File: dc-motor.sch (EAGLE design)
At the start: 82 parts, among them IC1 MEGA32-A, X3 RIA_3POL, X4 RIA_3POL, X5 RIA_2POL, X6 JUMP1-4, X8 PFVERB10

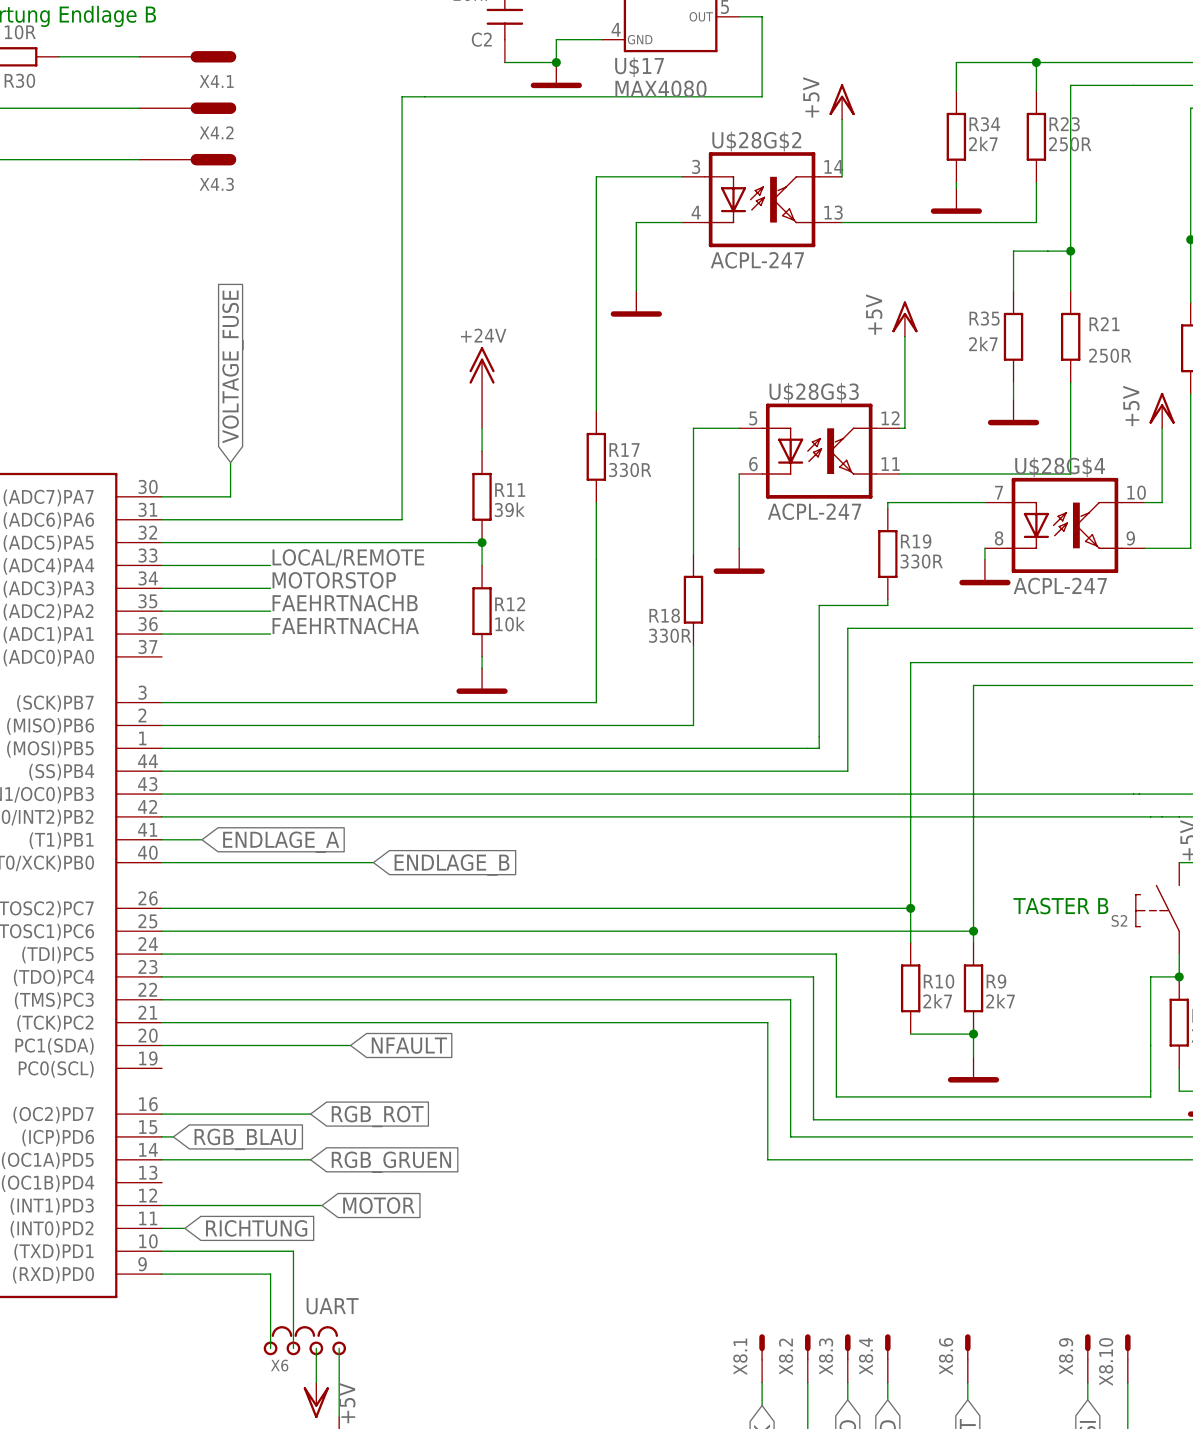
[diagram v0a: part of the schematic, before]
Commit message: edited again
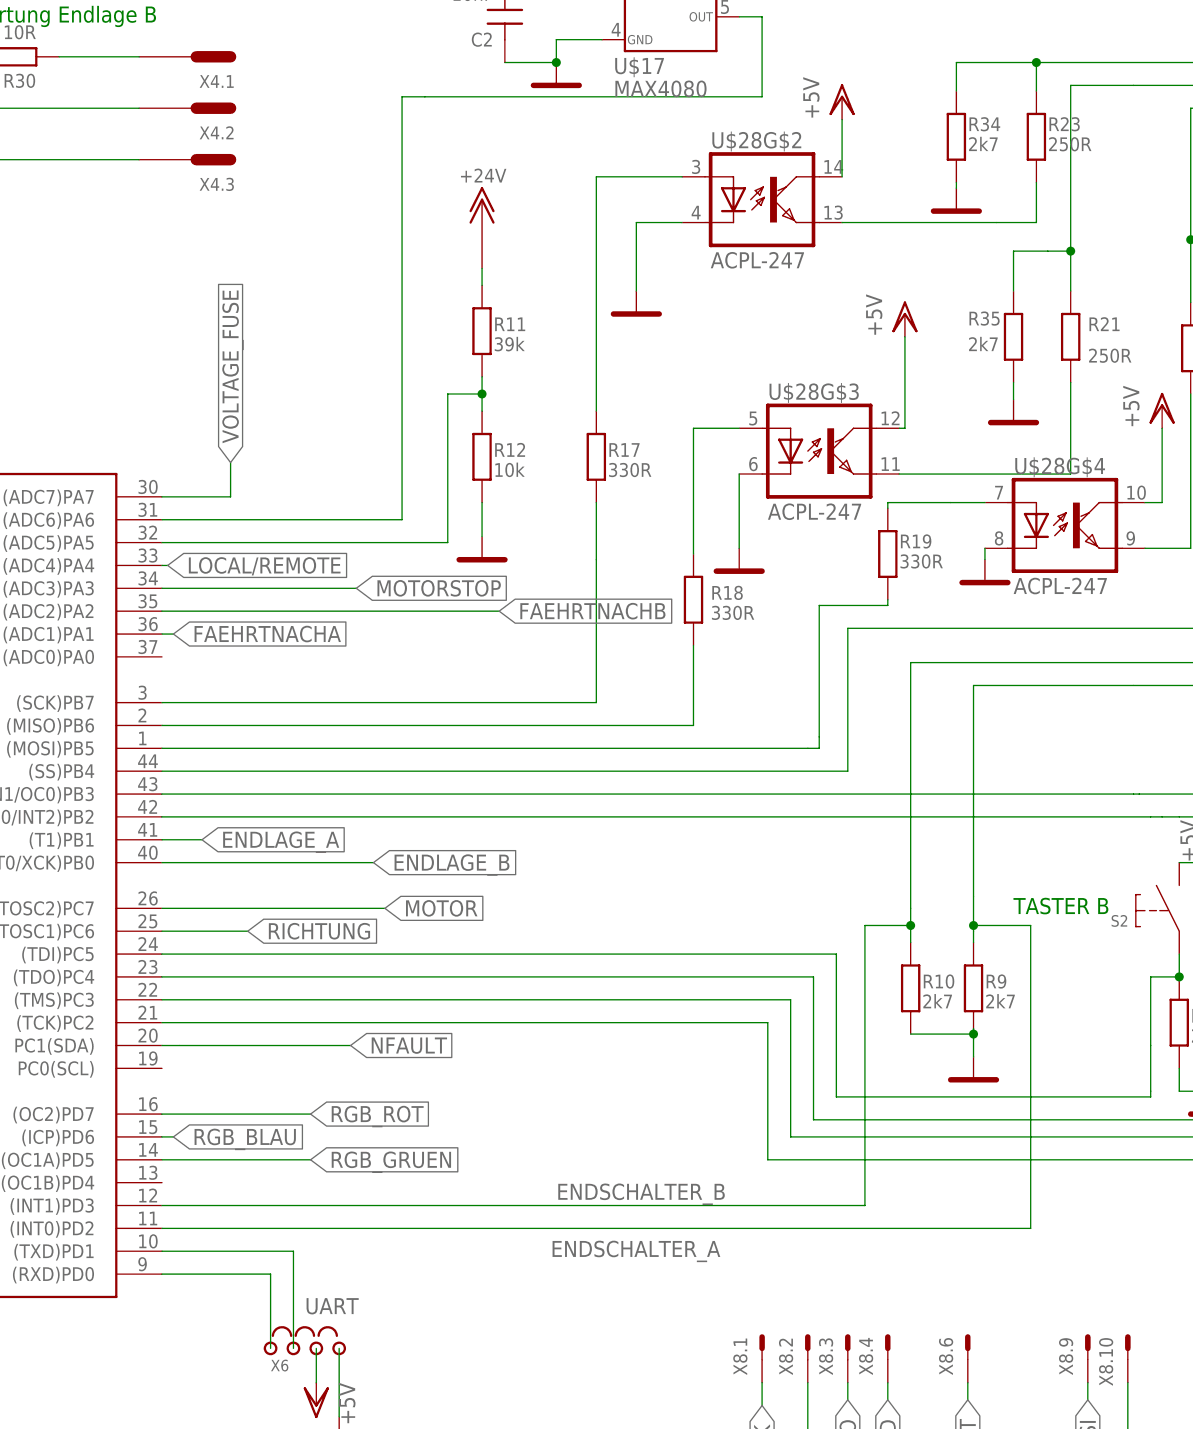
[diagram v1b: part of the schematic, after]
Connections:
- net ENDSCHALTER_A: now also IC1.(INT0)PD2; no longer IC1.(TOSC1)PC6
- net ENDSCHALTER_B: now also IC1.(INT1)PD3; no longer IC1.(TOSC2)PC7
- net MOTOR: now also IC1.(TOSC2)PC7; no longer IC1.(INT1)PD3
- net RICHTUNG: now also IC1.(TOSC1)PC6; no longer IC1.(INT0)PD2
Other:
- moved on the sheet: R11, R12
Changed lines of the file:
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@@
 </instance>
 <instance part="U$25" gate="G$1" x="288.29" y="191.135"/>
-<instance part="R11" gate="G$1" x="141.605" y="127" smashed="yes" rot="R90">
-<attribute name="NAME" x="142.875" y="127" size="1.524" layer="95"/>
-<attribute name="VALUE" x="142.875" y="124.7775" size="1.524" layer="96"/>
-</instance>
-<instance part="R12" gate="G$1" x="141.605" y="114.3" smashed="yes" rot="R90">
-<attribute name="NAME" x="142.875" y="114.3" size="1.524" layer="95"/>
-<attribute name="VALUE" x="142.875" y="112.0775" size="1.524" layer="96"/>
-</instance>
-<instance part="U$26" gate="G$1" x="141.605" y="105.41"/>
-<instance part="U$27" gate="G$1" x="141.605" y="137.16"/>
+<instance part="R11" gate="G$1" x="141.605" y="145.415" smashed="yes" rot="R90">
+<attribute name="NAME" x="142.875" y="145.415" size="1.524" layer="95"/>
+<attribute name="VALUE" x="142.875" y="143.1925" size="1.524" layer="96"/>
+</instance>
+<instance part="R12" gate="G$1" x="141.605" y="131.445" smashed="yes" rot="R90">
+<attribute name="NAME" x="142.875" y="131.445" size="1.524" layer="95"/>
+<attribute name="VALUE" x="142.875" y="129.2225" size="1.524" layer="96"/>
+</instance>
+<instance part="U$26" gate="G$1" x="141.605" y="120.015"/>
+<instance part="U$27" gate="G$1" x="141.605" y="154.94"/>
 <instance part="R14" gate="G$1" x="307.975" y="181.61" smashed="yes" rot="R90">
 <attribute name="NAME" x="309.245" y="181.61" size="1.524" layer="95"/>
@@
 </instance>
 <instance part="R18" gate="G$1" x="165.1" y="115.57" smashed="yes" rot="R270">
-<attribute name="NAME" x="160.02" y="113.03" size="1.524" layer="95"/>
-<attribute name="VALUE" x="160.02" y="110.8075" size="1.524" layer="96"/>
+<attribute name="NAME" x="167.005" y="115.57" size="1.524" layer="95"/>
+<attribute name="VALUE" x="167.005" y="113.3475" size="1.524" layer="96"/>
 </instance>
 <instance part="R19" gate="G$1" x="186.69" y="120.65" smashed="yes" rot="R90">
@@
 <pinref part="R12" gate="G$1" pin="1"/>
 <pinref part="U$26" gate="G$1" pin="GND"/>
-<wire x1="141.605" y1="109.22" x2="141.605" y2="107.95" width="0.1524" layer="91"/>
+<wire x1="141.605" y1="126.365" x2="141.605" y2="122.555" width="0.1524" layer="91"/>
 </segment>
 <segment>
@@
 <segment>
 <pinref part="R11" gate="G$1" pin="2"/>
-<wire x1="141.605" y1="132.08" x2="141.605" y2="134.62" width="0.1524" layer="91"/>
+<wire x1="141.605" y1="150.495" x2="141.605" y2="152.4" width="0.1524" layer="91"/>
 <pinref part="U$27" gate="G$1" pin="+24V"/>
 </segment>
@@
 <pinref part="R9" gate="G$1" pin="2"/>
 <wire x1="196.215" y1="77.47" x2="196.215" y2="78.74" width="0.1524" layer="91"/>
-<wire x1="196.215" y1="78.74" x2="196.215" y2="82.55" width="0.1524" layer="91"/>
+<wire x1="196.215" y1="78.74" x2="196.215" y2="79.375" width="0.1524" layer="91"/>
+<wire x1="196.215" y1="79.375" x2="196.215" y2="82.55" width="0.1524" layer="91"/>
 <wire x1="196.215" y1="82.55" x2="196.215" y2="106.045" width="0.1524" layer="91"/>
 <wire x1="196.215" y1="106.045" x2="213.995" y2="106.045" width="0.1524" layer="91"/>
 <wire x1="213.995" y1="106.045" x2="343.535" y2="106.045" width="0.1524" layer="91"/>
-<pinref part="IC1" gate="G$1" pin="(TOSC1)PC6"/>
-<wire x1="106.045" y1="78.74" x2="196.215" y2="78.74" width="0.1524" layer="91"/>
-<junction x="196.215" y="78.74"/>
 <pinref part="X1" gate="G$1" pin="3"/>
 <wire x1="343.535" y1="170.18" x2="345.44" y2="170.18" width="0.1524" layer="91"/>
@@
 <wire x1="343.535" y1="106.045" x2="343.535" y2="170.18" width="0.1524" layer="91"/>
 <label x="316.865" y="255.27" size="1.778" layer="95" font="vector" rot="R180" xref="yes"/>
+<pinref part="IC1" gate="G$1" pin="(INT0)PD2"/>
+<wire x1="106.045" y1="45.72" x2="202.565" y2="45.72" width="0.1524" layer="91"/>
+<wire x1="202.565" y1="45.72" x2="202.565" y2="79.375" width="0.1524" layer="91"/>
+<wire x1="202.565" y1="79.375" x2="196.215" y2="79.375" width="0.1524" layer="91"/>
+<junction x="196.215" y="79.375"/>
+<label x="149.225" y="42.545" size="1.778" layer="95"/>
 </segment>
 <segment>
@@
 <pinref part="R10" gate="G$1" pin="2"/>
 <wire x1="189.23" y1="108.585" x2="189.23" y2="81.28" width="0.1524" layer="91"/>
-<wire x1="189.23" y1="81.28" x2="189.23" y2="77.47" width="0.1524" layer="91"/>
+<wire x1="189.23" y1="81.28" x2="189.23" y2="79.375" width="0.1524" layer="91"/>
+<wire x1="189.23" y1="79.375" x2="189.23" y2="77.47" width="0.1524" layer="91"/>
 <wire x1="189.23" y1="108.585" x2="340.995" y2="108.585" width="0.1524" layer="91"/>
 <wire x1="340.995" y1="108.585" x2="340.995" y2="133.985" width="0.1524" layer="91"/>
-<pinref part="IC1" gate="G$1" pin="(TOSC2)PC7"/>
-<wire x1="106.045" y1="81.28" x2="189.23" y2="81.28" width="0.1524" layer="91"/>
-<junction x="189.23" y="81.28"/>
 <pinref part="X1" gate="G$1" pin="2"/>
 <wire x1="346.075" y1="172.72" x2="343.535" y2="172.72" width="0.1524" layer="91"/>
@@
 <wire x1="340.995" y1="133.985" x2="340.995" y2="172.72" width="0.1524" layer="91"/>
 <label x="319.405" y="249.555" size="1.778" layer="95" font="vector" rot="R180" xref="yes"/>
+<pinref part="IC1" gate="G$1" pin="(INT1)PD3"/>
+<wire x1="106.045" y1="48.26" x2="184.15" y2="48.26" width="0.1524" layer="91"/>
+<wire x1="184.15" y1="48.26" x2="184.15" y2="79.375" width="0.1524" layer="91"/>
+<wire x1="184.15" y1="79.375" x2="189.23" y2="79.375" width="0.1524" layer="91"/>
+<junction x="189.23" y="79.375"/>
+<label x="149.86" y="48.895" size="1.778" layer="95"/>
 </segment>
 <segment>
@@
 <wire x1="293.37" y1="149.86" x2="280.67" y2="149.86" width="0.1524" layer="91"/>
 <junction x="280.67" y="149.86"/>
-</segment>
-</net>
-<net name="N$50" class="0">
-<segment>
-<pinref part="R11" gate="G$1" pin="1"/>
-<pinref part="R12" gate="G$1" pin="2"/>
-<wire x1="141.605" y1="119.38" x2="141.605" y2="121.92" width="0.1524" layer="91"/>
-<wire x1="141.605" y1="121.92" x2="140.97" y2="121.92" width="0.1524" layer="91"/>
-<junction x="141.605" y="121.92"/>
-<wire x1="140.97" y1="121.92" x2="140.335" y2="121.92" width="0.1524" layer="91"/>
-<pinref part="IC1" gate="G$1" pin="(ADC5)PA5"/>
-<wire x1="106.045" y1="121.92" x2="138.43" y2="121.92" width="0.1524" layer="91"/>
-<wire x1="138.43" y1="121.92" x2="140.335" y2="121.92" width="0.1524" layer="91"/>
 </segment>
 </net>
@@
 <segment>
 <pinref part="IC1" gate="G$1" pin="(ADC4)PA4"/>
-<wire x1="106.045" y1="119.38" x2="118.11" y2="119.38" width="0.1524" layer="91"/>
-<label x="118.11" y="119.38" size="1.778" layer="95" font="vector"/>
+<wire x1="106.045" y1="119.38" x2="106.68" y2="119.38" width="0.1524" layer="91"/>
+<label x="106.68" y="119.38" size="1.778" layer="95" font="vector" xref="yes"/>
 </segment>
 <segment>
@@
 <segment>
 <pinref part="IC1" gate="G$1" pin="(ADC3)PA3"/>
-<wire x1="106.045" y1="116.84" x2="118.11" y2="116.84" width="0.1524" layer="91"/>
-<label x="118.11" y="116.84" size="1.778" layer="95" font="vector"/>
+<wire x1="106.045" y1="116.84" x2="127.635" y2="116.84" width="0.1524" layer="91"/>
+<label x="127.635" y="116.84" size="1.778" layer="95" font="vector" xref="yes"/>
 </segment>
 </net>
@@
 <segment>
 <pinref part="IC1" gate="G$1" pin="(ADC2)PA2"/>
-<wire x1="118.11" y1="114.3" x2="106.045" y2="114.3" width="0.1524" layer="91"/>
-<label x="118.11" y="114.3" size="1.778" layer="95" font="vector"/>
+<wire x1="143.51" y1="114.3" x2="106.045" y2="114.3" width="0.1524" layer="91"/>
+<label x="143.51" y="114.3" size="1.778" layer="95" font="vector" xref="yes"/>
 </segment>
 </net>
@@
 <segment>
 <pinref part="IC1" gate="G$1" pin="(ADC1)PA1"/>
-<wire x1="106.045" y1="111.76" x2="118.11" y2="111.76" width="0.1524" layer="91"/>
-<label x="118.11" y="111.76" size="1.778" layer="95" font="vector"/>
+<wire x1="106.045" y1="111.76" x2="107.315" y2="111.76" width="0.1524" layer="91"/>
+<label x="107.315" y="111.76" size="1.778" layer="95" font="vector" xref="yes"/>
 </segment>
 <segment>
@@
 <net name="RICHTUNG" class="0">
 <segment>
-<pinref part="IC1" gate="G$1" pin="(INT0)PD2"/>
-<wire x1="106.045" y1="45.72" x2="108.585" y2="45.72" width="0.1524" layer="91"/>
-<label x="108.585" y="45.72" size="1.778" layer="95" font="vector" xref="yes"/>
-</segment>
-<segment>
 <pinref part="X1" gate="G$1" pin="9"/>
 <wire x1="361.315" y1="165.1" x2="361.95" y2="165.1" width="0.1524" layer="91"/>
 <label x="361.95" y="165.1" size="1.778" layer="95" font="vector" xref="yes"/>
 </segment>
+<segment>
+<pinref part="IC1" gate="G$1" pin="(TOSC1)PC6"/>
+<wire x1="115.57" y1="78.74" x2="106.045" y2="78.74" width="0.1524" layer="91"/>
+<label x="115.57" y="78.74" size="1.778" layer="95" xref="yes"/>
+</segment>
 </net>
 <net name="MOTOR" class="0">
-<segment>
-<pinref part="IC1" gate="G$1" pin="(INT1)PD3"/>
-<wire x1="106.045" y1="48.26" x2="123.825" y2="48.26" width="0.1524" layer="91"/>
-<label x="123.825" y="48.26" size="1.778" layer="95" font="vector" xref="yes"/>
-</segment>
 <segment>
 <pinref part="X1" gate="G$1" pin="6"/>
@@
 <label x="361.95" y="172.72" size="1.778" layer="95" font="vector" xref="yes"/>
 </segment>
+<segment>
+<pinref part="IC1" gate="G$1" pin="(TOSC2)PC7"/>
+<wire x1="106.045" y1="81.28" x2="130.81" y2="81.28" width="0.1524" layer="91"/>
+<label x="130.81" y="81.28" size="1.778" layer="95" xref="yes"/>
+</segment>
 </net>
 <net name="RGB_ROT" class="0">
@@
 </segment>
 </net>
+<net name="N$20" class="0">
+<segment>
+<pinref part="R11" gate="G$1" pin="1"/>
+<pinref part="R12" gate="G$1" pin="2"/>
+<wire x1="141.605" y1="136.525" x2="141.605" y2="138.43" width="0.1524" layer="91"/>
+<wire x1="141.605" y1="138.43" x2="141.605" y2="140.335" width="0.1524" layer="91"/>
+<pinref part="IC1" gate="G$1" pin="(ADC5)PA5"/>
+<wire x1="106.045" y1="121.92" x2="137.795" y2="121.92" width="0.1524" layer="91"/>
+<wire x1="141.605" y1="138.43" x2="137.795" y2="138.43" width="0.1524" layer="91"/>
+<wire x1="137.795" y1="138.43" x2="137.795" y2="121.92" width="0.1524" layer="91"/>
+<junction x="141.605" y="138.43"/>
+</segment>
+</net>
